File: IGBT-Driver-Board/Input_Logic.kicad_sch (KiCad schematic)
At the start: 15 parts, among them U2 MGJ2D051515SC

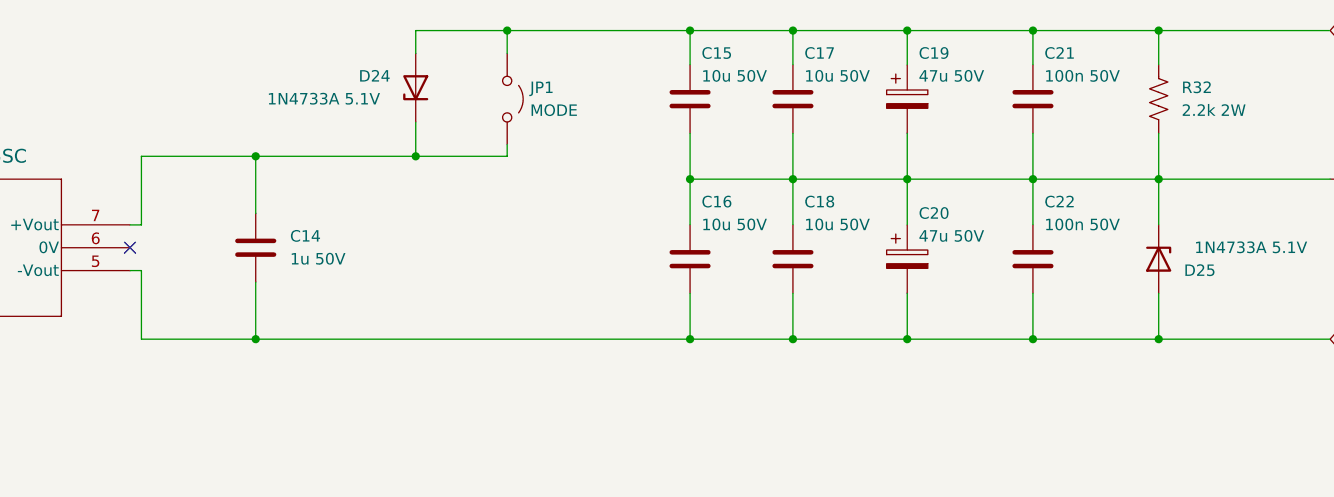
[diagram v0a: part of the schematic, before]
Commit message: version 2.0.0
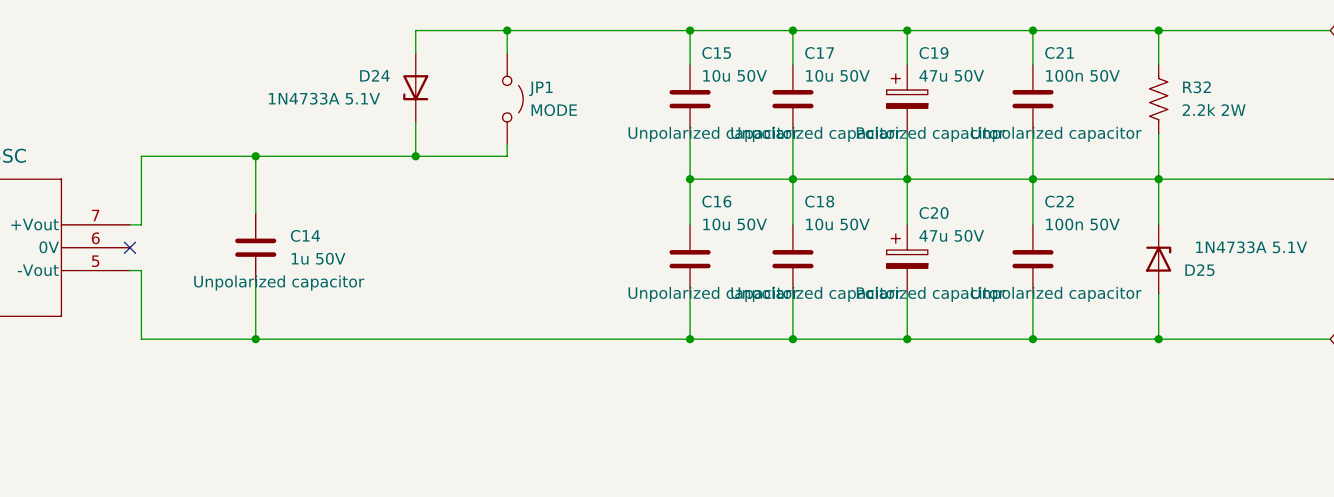
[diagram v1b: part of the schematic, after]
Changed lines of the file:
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@@
 			)
 		)
-		(property "Description" ""
+		(property "Description" "Unpolarized capacitor"
 			(at 204.47 109.22 0)
 			(show_name no)
@@
 			)
 		)
-		(property "Description" ""
+		(property "Description" "Polarized capacitor"
 			(at 190.5 109.22 0)
 			(show_name no)
@@
 			)
 		)
-		(property "Description" ""
+		(property "Description" "Polarized capacitor"
 			(at 190.5 91.44 0)
 			(show_name no)
@@
 			)
 		)
-		(property "Description" ""
+		(property "Description" "Unpolarized capacitor"
 			(at 118.11 107.95 0)
 			(show_name no)
@@
 			)
 		)
-		(property "Description" ""
+		(property "Description" "Unpolarized capacitor"
 			(at 177.8 91.44 0)
 			(show_name no)
@@
 			)
 		)
-		(property "Description" ""
+		(property "Description" "Unpolarized capacitor"
 			(at 204.47 91.44 0)
 			(show_name no)
@@
 			)
 		)
-		(property "Description" ""
+		(property "Description" "Unpolarized capacitor"
 			(at 166.37 91.44 0)
 			(show_name no)
@@
 			)
 		)
-		(property "Description" ""
+		(property "Description" "Unpolarized capacitor"
 			(at 166.37 109.22 0)
 			(show_name no)
@@
 			)
 		)
-		(property "Description" ""
+		(property "Description" "Unpolarized capacitor"
 			(at 177.8 109.22 0)
 			(show_name no)
